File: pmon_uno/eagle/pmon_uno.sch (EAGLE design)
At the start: 42 parts, among them J1 USB, J2 USB, J3 TERMINAL-2, Q1 16Mhz, U1 LTC2943, U2 FT232RL, U3 LT1764AEQ, U4 ATMEGA328TQFP32

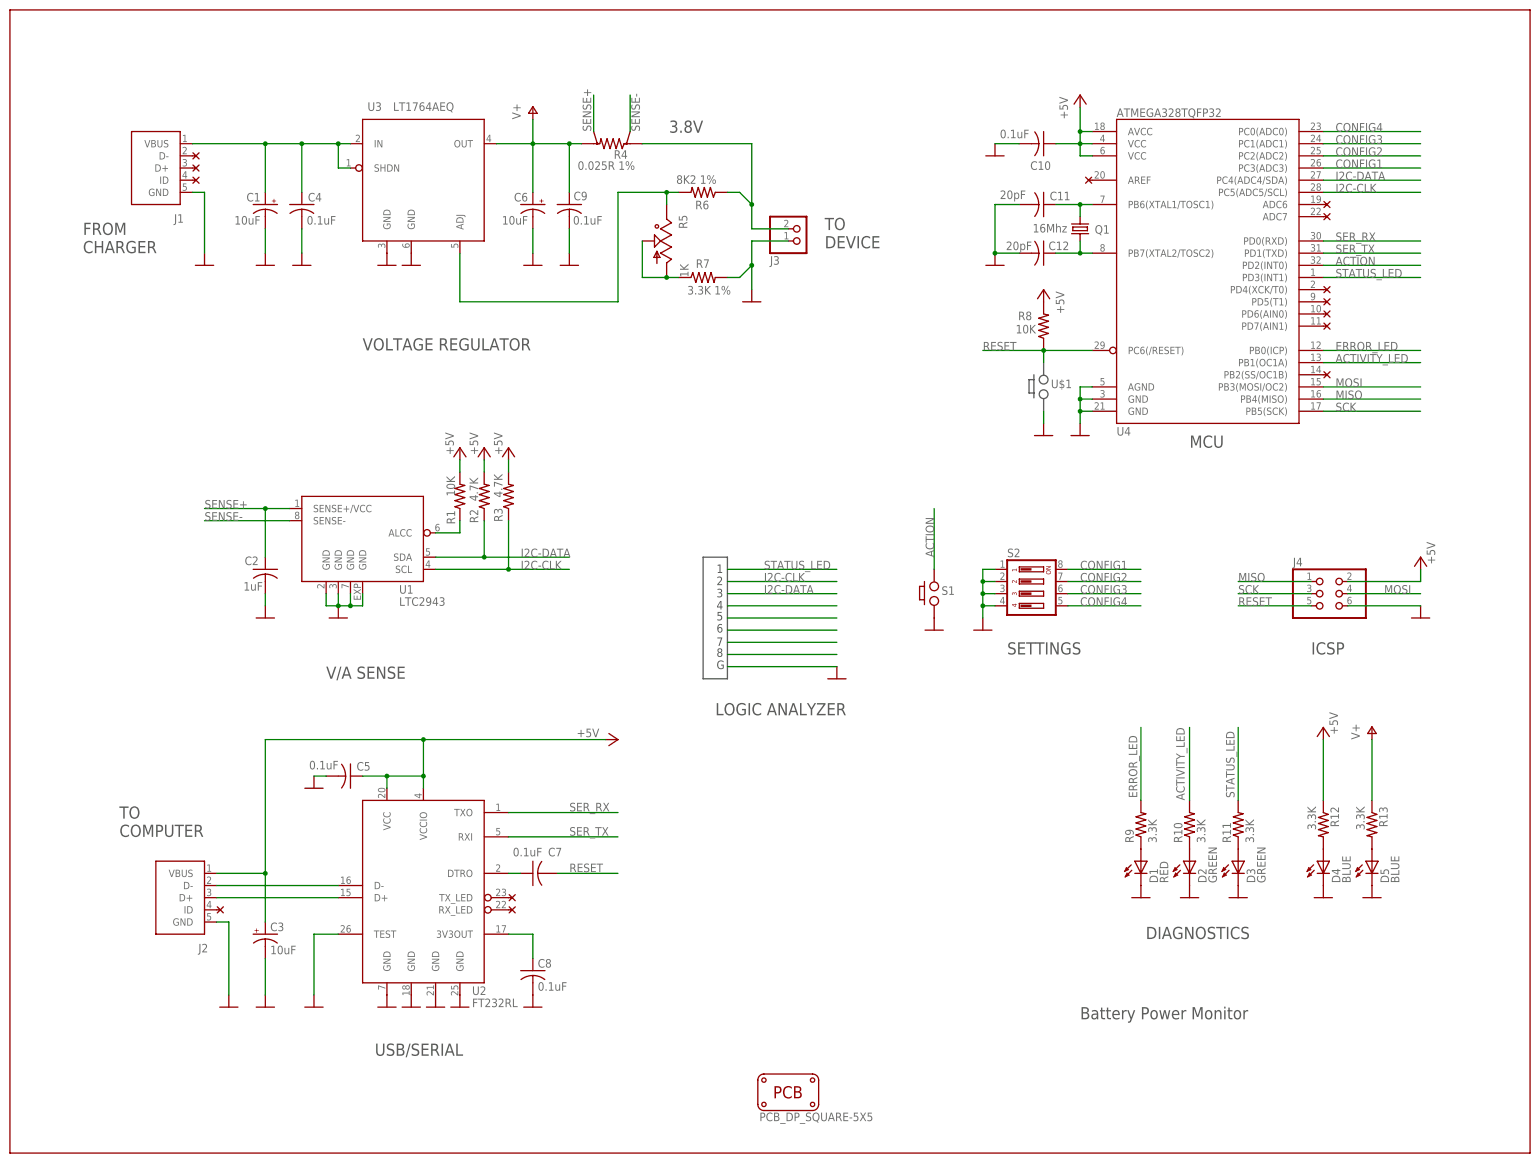
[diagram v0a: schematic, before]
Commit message: Layout completed.
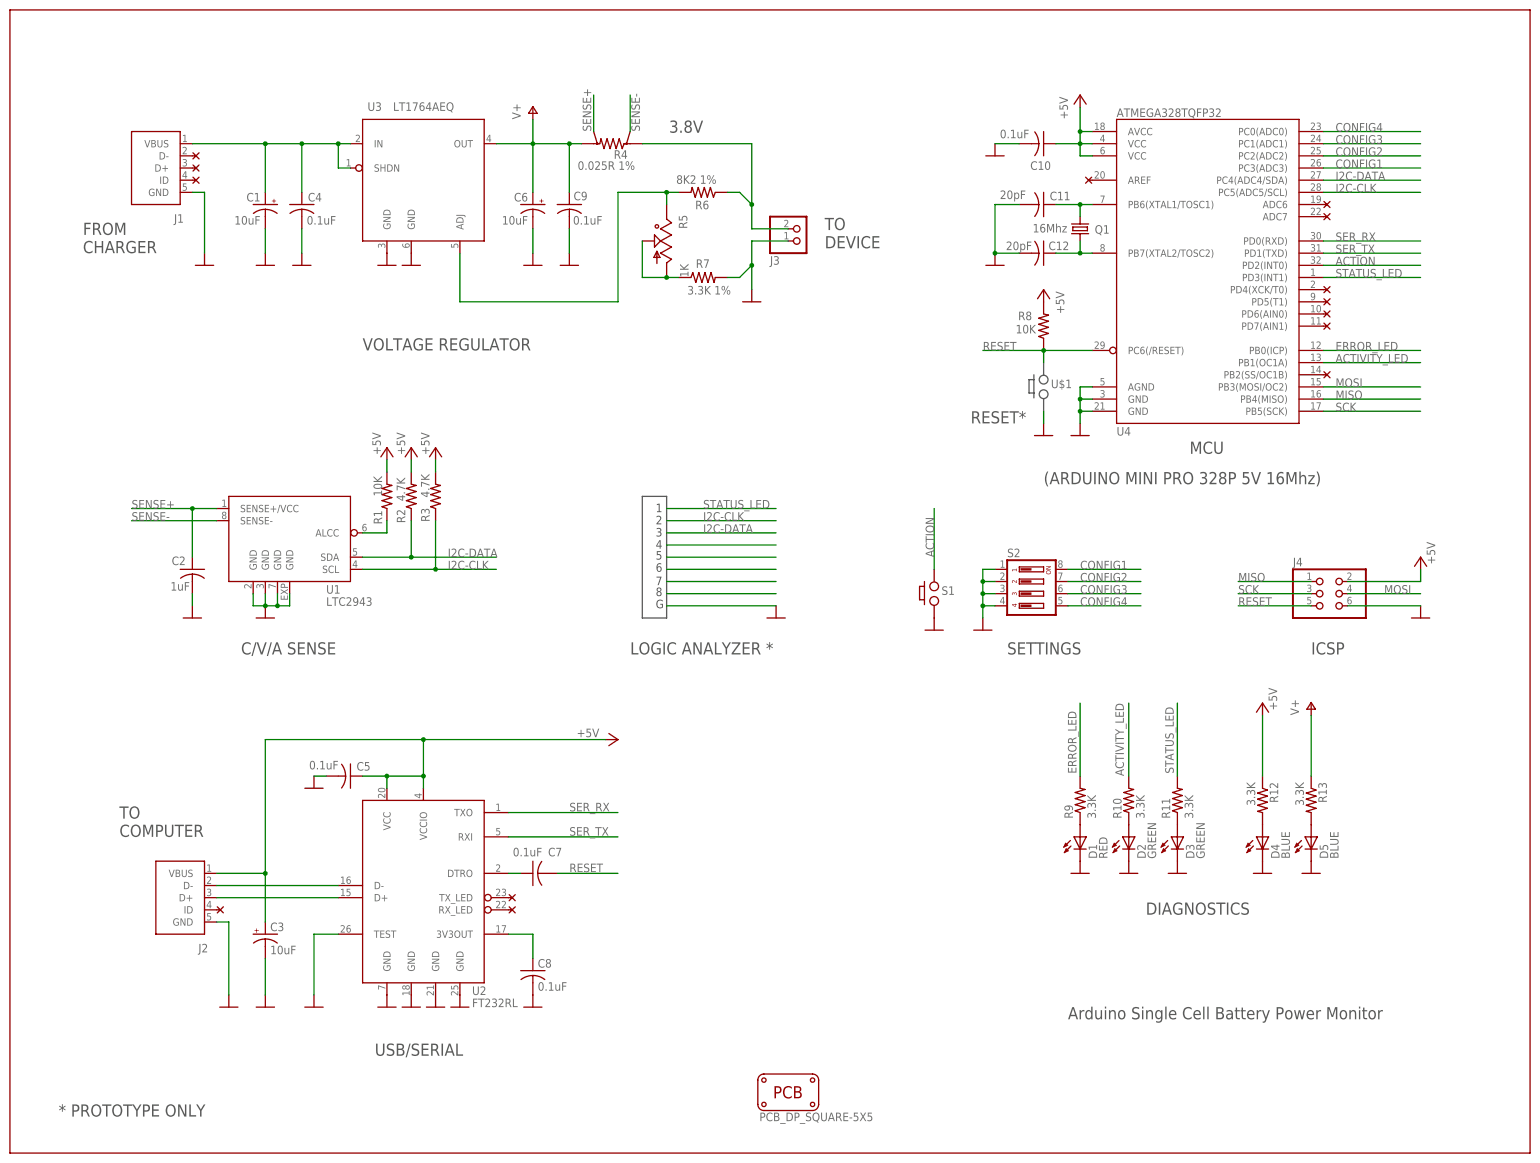
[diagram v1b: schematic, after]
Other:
- note added: "(ARDUINO MINI PRO 328P 5V 16Mhz)"
- note added: "* PROTOTYPE ONLY"
- note added: "Arduino Single Cell Battery Power Monitor"
- note added: "C/V/A SENSE"
- note added: "LOGIC ANALYZER *"
- note added: "RESET*"
- note removed: "Battery Power Monitor"
- note removed: "LOGIC ANALYZER"
- note removed: "V/A SENSE"
- moved on the sheet: C2, D1, D2, D3, D4, D5, R1, R10, R11, R12, R13, R2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
